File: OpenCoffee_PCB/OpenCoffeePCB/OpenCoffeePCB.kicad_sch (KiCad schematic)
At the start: 3 parts, among them U1 Pico, U2 Pico_WiFi

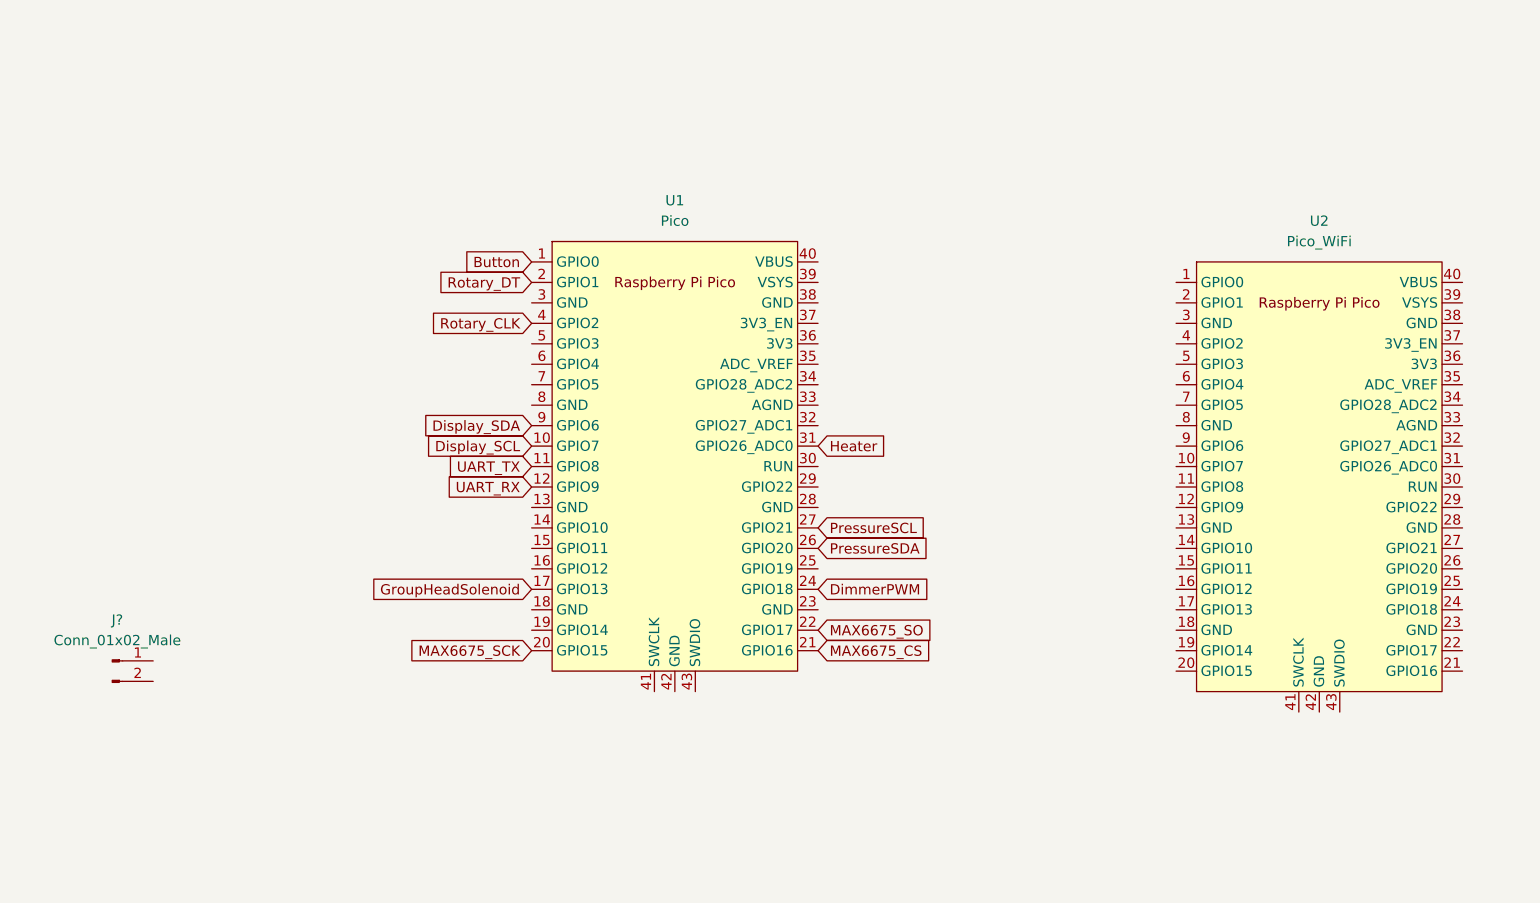
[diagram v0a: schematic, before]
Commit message: intial layout
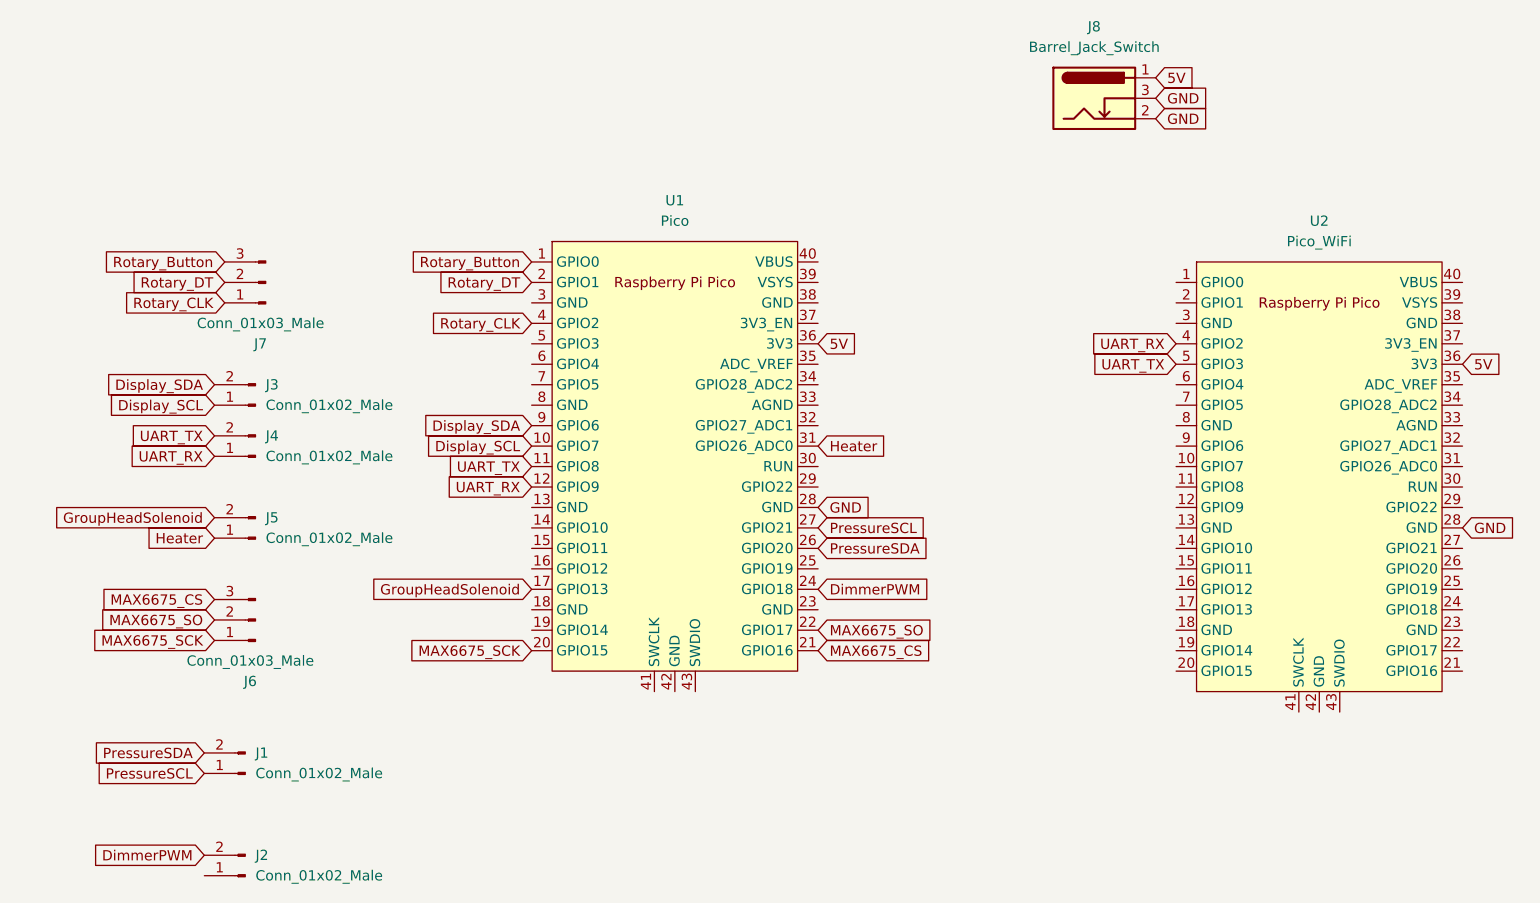
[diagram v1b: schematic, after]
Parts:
- removed J?: Conn_01x02_Male, symbol Connector:Conn_01x02_Male
- added J1, J2, J3, J4, J5: Conn_01x02_Male, Connector_Molex:Molex_KK-254_AE-6410-03A_1x03_P2.54mm_Vertical, symbol Connector:Conn_01x02_Male
- added J6, J7: Conn_01x03_Male, Connector_Molex:Molex_KK-254_AE-6410-03A_1x03_P2.54mm_Vertical, symbol Connector:Conn_01x03_Male
- added J8: Barrel_Jack_Switch, Connector_BarrelJack:BarrelJack_GCT_DCJ200-10-A_Horizontal, symbol Connector:Barrel_Jack_Switch
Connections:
- net DimmerPWM: now also J2.2 (Pin_2)
- net Display_SCL: now also J3.1 (Pin_1)
- net Display_SDA: now also J3.2 (Pin_2)
- net GroupHeadSolenoid: now also J5.2 (Pin_2)
- net Heater: now also J5.1 (Pin_1)
- net MAX6675_CS: now also J6.3 (Pin_3)
- net MAX6675_SCK: now also J6.1 (Pin_1)
- net MAX6675_SO: now also J6.2 (Pin_2)
- net PressureSCL: now also J1.1 (Pin_1)
- net PressureSDA: now also J1.2 (Pin_2)
- net Rotary_CLK: now also J7.1 (Pin_1)
- net Rotary_DT: now also J7.2 (Pin_2)
- net UART_RX: now also U2.4 (GPIO2), J4.1 (Pin_1)
- net UART_TX: now also U2.5 (GPIO3), J4.2 (Pin_2)
- net GND: now reaches U1.28 (GND)
- net GND: now also U2.28 (GND), J8.2, J8.3
- net 5V: now reaches U1.36 (3V3)
- net 5V: now also U2.36 (3V3), J8.1
- net Button renamed Rotary_Button
- net Rotary_Button: now also J7.3 (Pin_3)
